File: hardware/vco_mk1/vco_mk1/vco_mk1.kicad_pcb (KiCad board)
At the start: 2 copper layers, 50 x 80 mm, 88 parts, among them J1 power supply, J2 control in, J3 signal out, J4 Conn_01x03_Male, J5 BCM847 breakout socket, J6 Conn_01x01_Male, Q1 BCM847, Q2 BC547, Q3 BC547, Q4 2N7000, Q5 BC547, Q6 BC327, U1 LM324, U2 LM324, U3 74HC86

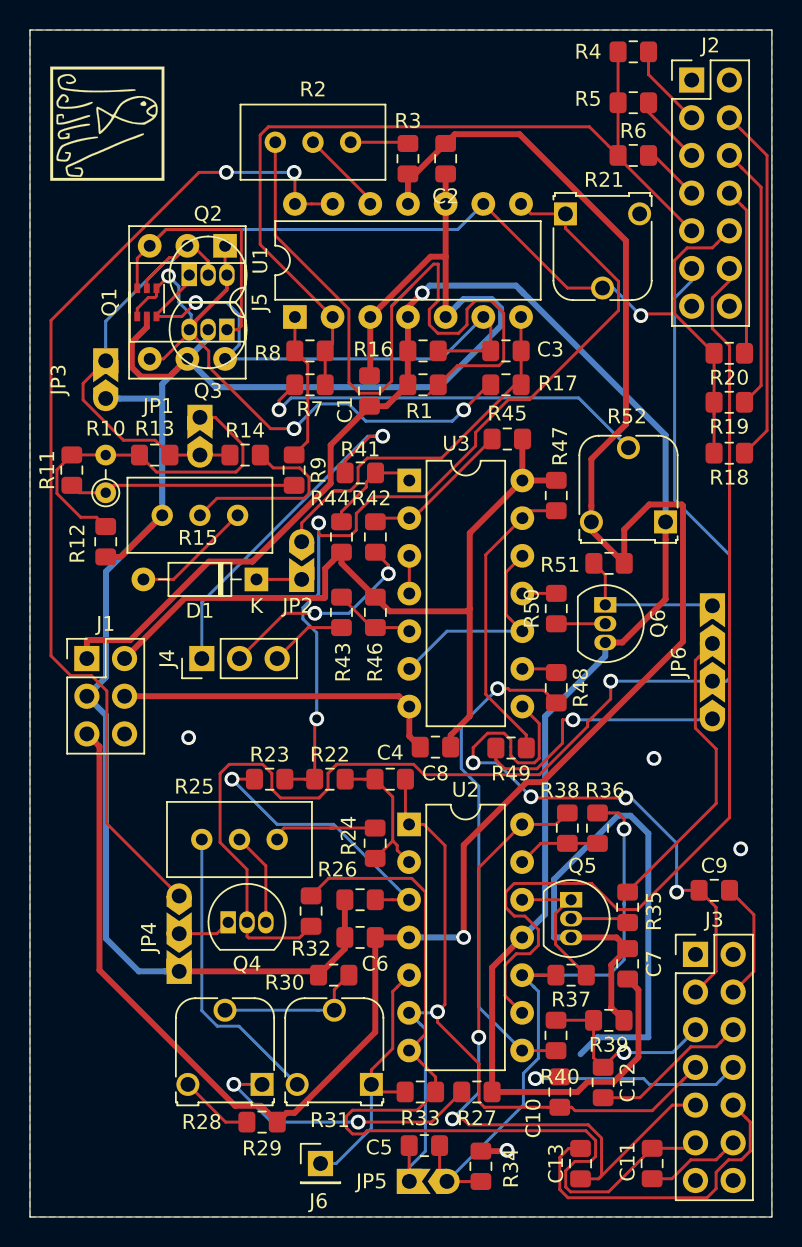
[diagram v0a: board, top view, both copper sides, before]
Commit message: clean slate reroute with cleaner layout
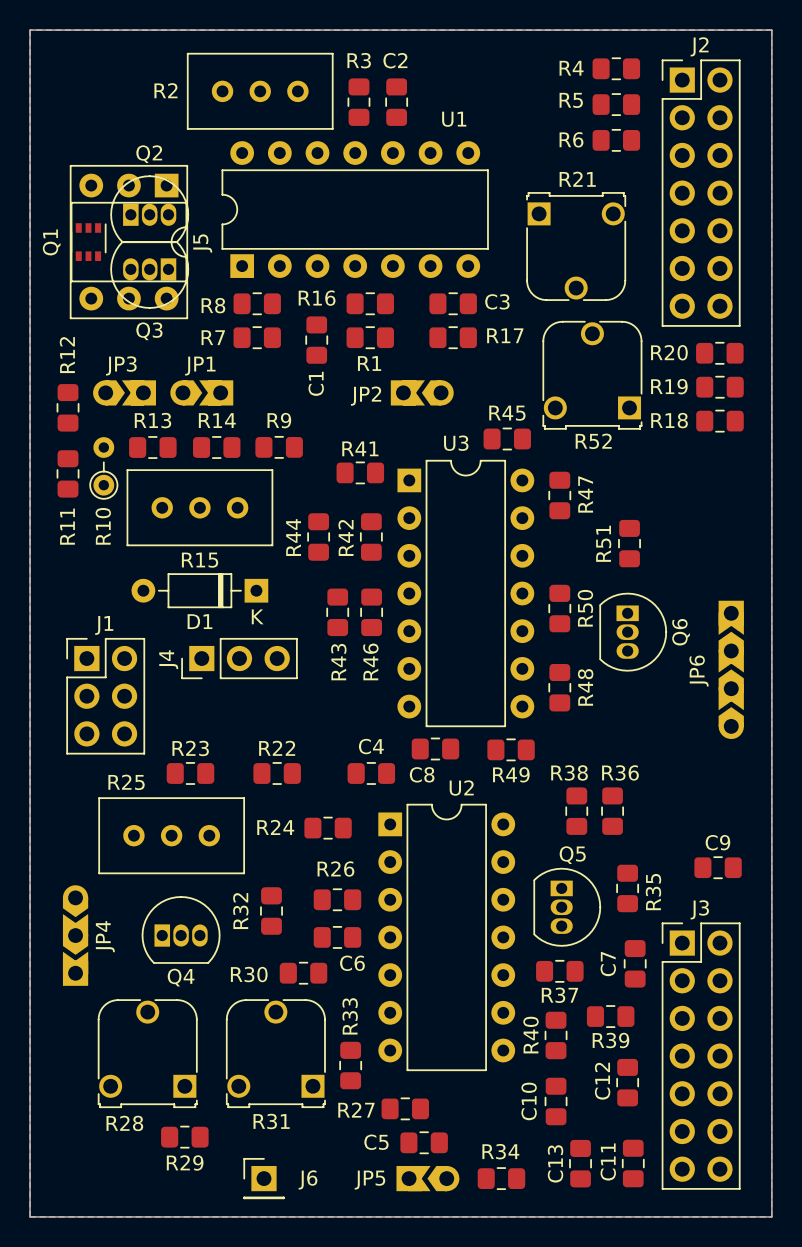
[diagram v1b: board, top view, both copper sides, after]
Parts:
- removed FISCH: LOGO, footprints:windfisch
- moved JP2 13.9 mm to (186.4, 84.5), turned to 0 degrees
- moved R12 9.38 mm to (162.6, 85.5), turned to 90 degrees
- moved R52 8.06 mm to (200.4, 85.5)
- moved JP4 6.99 mm to (163.1, 121.0)
- moved J5 5.66 mm to (169.2, 70.5)
- moved Q1 5.66 mm to (163.9, 74.3)
- moved Q3 5.66 mm to (169.3, 76.1)
- moved Q2 5.66 mm to (166.8, 72.4)
- moved R23 5.35 mm to (170.8, 110.1)
- moved R29 5.30 mm to (170.4, 134.6)
- moved R28 5.21 mm to (170.4, 131.2)
- moved R3 5.04 mm to (182.2, 64.9)
- moved C2 5.04 mm to (184.7, 64.9)
- moved R33 5.02 mm to (181.6, 129.8), turned to 90 degrees
- moved R27 4.96 mm to (185.3, 132.7)
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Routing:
- net GND: track 177.0 -> 0.00 mm, vias 4 -> 0
- net VEE: track 141.2 -> 0.00 mm, vias 1 -> 0
- net VCC: track 125.9 -> 0.00 mm, vias 1 -> 0
- net ctl_override: track 88.1 -> 0.00 mm, vias 1 -> 0
- net C2: track 75.9 -> 0.00 mm, vias 1 -> 0
- net var_vsource: track 68.4 -> 0.00 mm, vias 2 -> 0
- net V_pwm: track 68.0 -> 0.00 mm
- net square_ctl: track 63.0 -> 0.00 mm
- net V_expo: track 60.0 -> 0.00 mm, vias 2 -> 0
- net V_control_raw: track 58.3 -> 0.00 mm
- net triangle: track 57.5 -> 0.00 mm, vias 1 -> 0
- net +5V: track 54.6 -> 0.00 mm
- net Net-(R1-Pad2): track 53.6 -> 0.00 mm
- net E: track 49.4 -> 0.00 mm, vias 3 -> 0
- net sawtooth: track 49.0 -> 0.00 mm, vias 2 -> 0
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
